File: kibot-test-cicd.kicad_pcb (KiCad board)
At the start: 4 copper layers, 47 x 47 mm, 12 parts, among them J1 Conn_02x04_Counter_Clockwise, J2 Conn_01x05_Pin, U1 MT6701CT

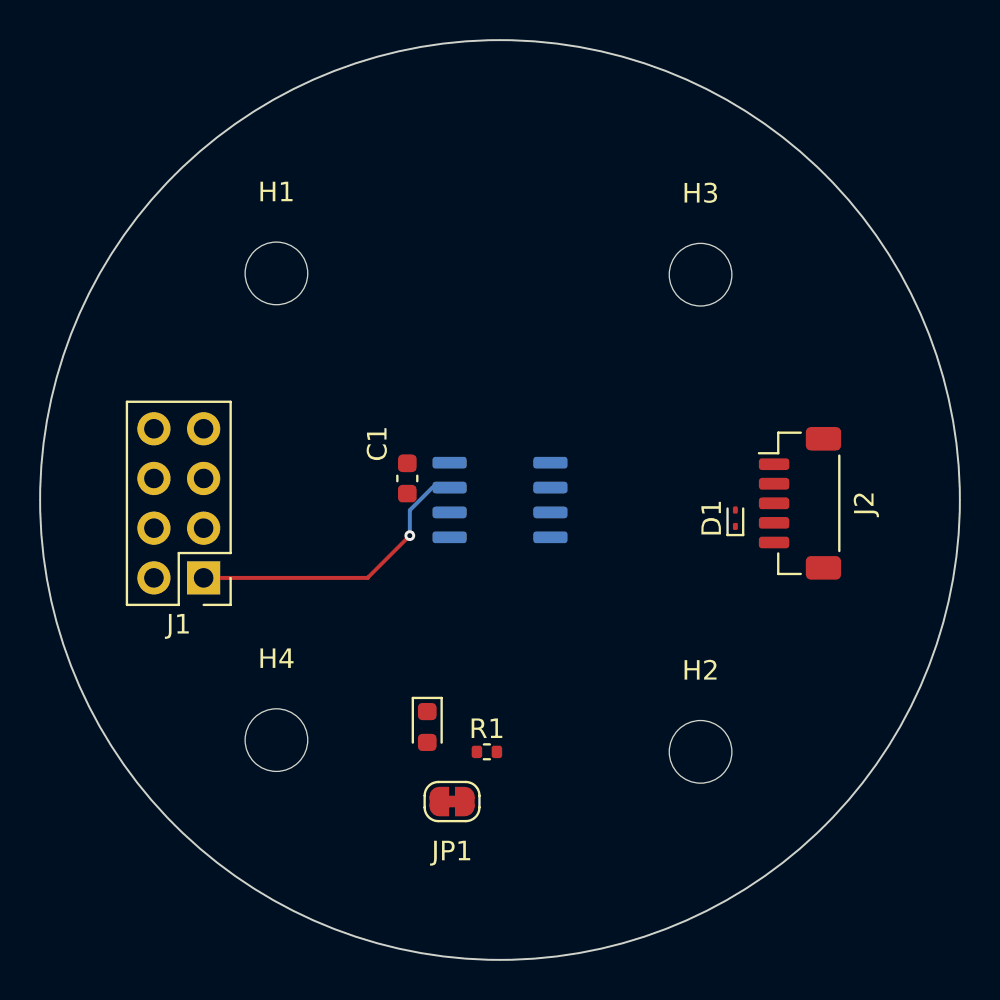
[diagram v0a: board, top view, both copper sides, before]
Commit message: [PCB] finished layout
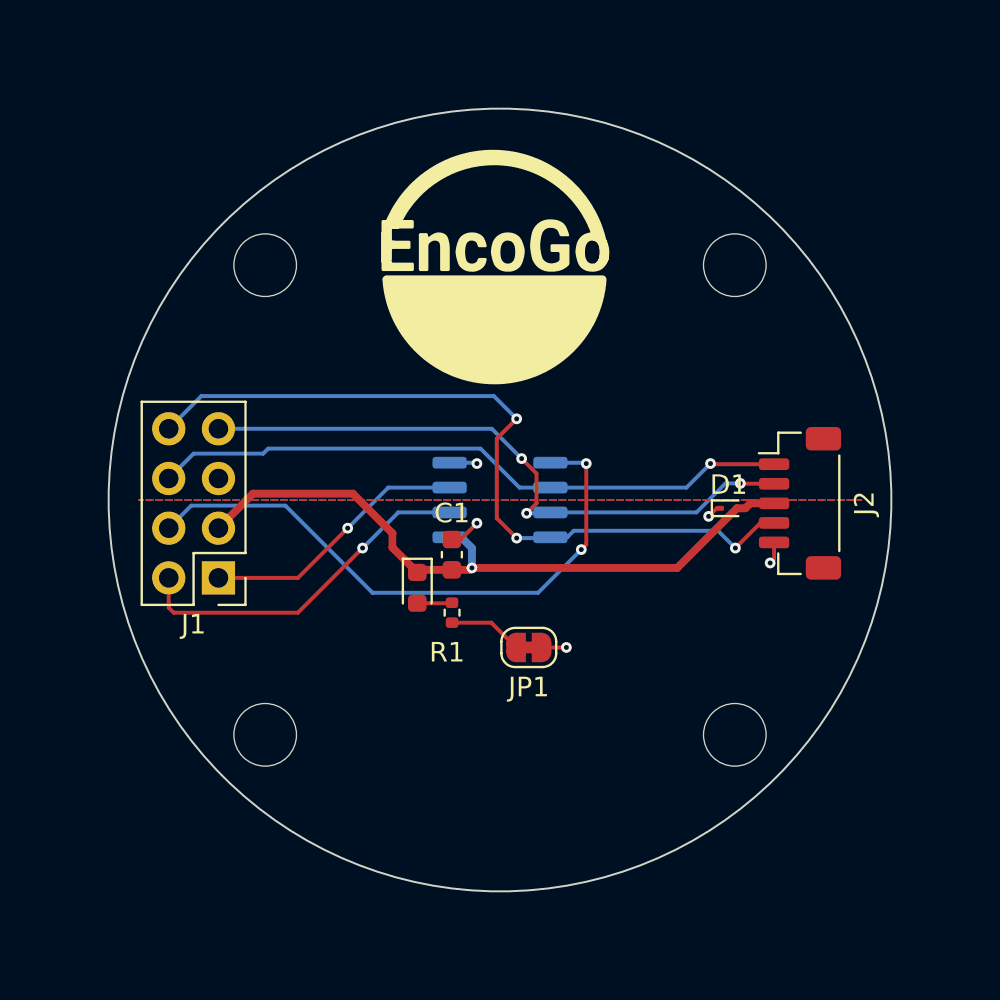
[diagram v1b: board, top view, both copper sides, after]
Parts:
- moved JP1 8.80 mm to (150.0, 97.5), turned to 180 degrees
- moved R1 7.33 mm to (146.1, 95.8), turned to -90 degrees
- moved D2 7.13 mm to (144.3, 94.5)
- moved C1 4.51 mm to (146.0, 92.8), turned to 90 degrees
- moved H2 1.95 mm to (160.5, 102.0)
- moved H3 1.82 mm to (160.5, 78.0)
- moved J1 0.76 mm to (134.1, 94.0)
- moved H1 0.71 mm to (136.5, 78.0)
- moved H4 0.64 mm to (136.5, 102.0)
- moved D1 0.61 mm to (160.2, 90.4), turned to 0 degrees
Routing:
- net Z-CS: track 0.00 -> 40.1 mm, vias 0 -> 3
- net +3V3: track 0.00 -> 35.3 mm, vias 0 -> 1
- net SDA-A: track 0.00 -> 32.9 mm, vias 0 -> 1
- net SCL-B: track 0.00 -> 32.7 mm, vias 0 -> 3
- net push: track 0.00 -> 30.7 mm, vias 0 -> 2
- net mode: track 0.00 -> 18.1 mm, vias 0 -> 1
- net GND: track 0.00 -> 6.21 mm, vias 0 -> 5
- net Net-(JP1-B): track 0.00 -> 3.80 mm
- net Net-(D2-A): track 0.00 -> 1.79 mm
- net out_sel: track 15.4 -> 13.7 mm
- added copper zone on B.Cu, net GND
- added copper zone on F.Cu, net GND
- removed copper zone on In1.Cu, net (none)
- removed copper zone on In2.Cu, net (none)
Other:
- board size 47 x 47 mm -> 40 x 40 mm
- copper layers 4 -> 2

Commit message: minor adjustments
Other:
- board text added: "4x M3"
- board text added: "R 20"
